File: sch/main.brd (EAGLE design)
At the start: 99.1 x 50.8 mm, 24 parts, among them IC2 PIC16F628P, T1 BC337, T2 BC337, T3 BC337

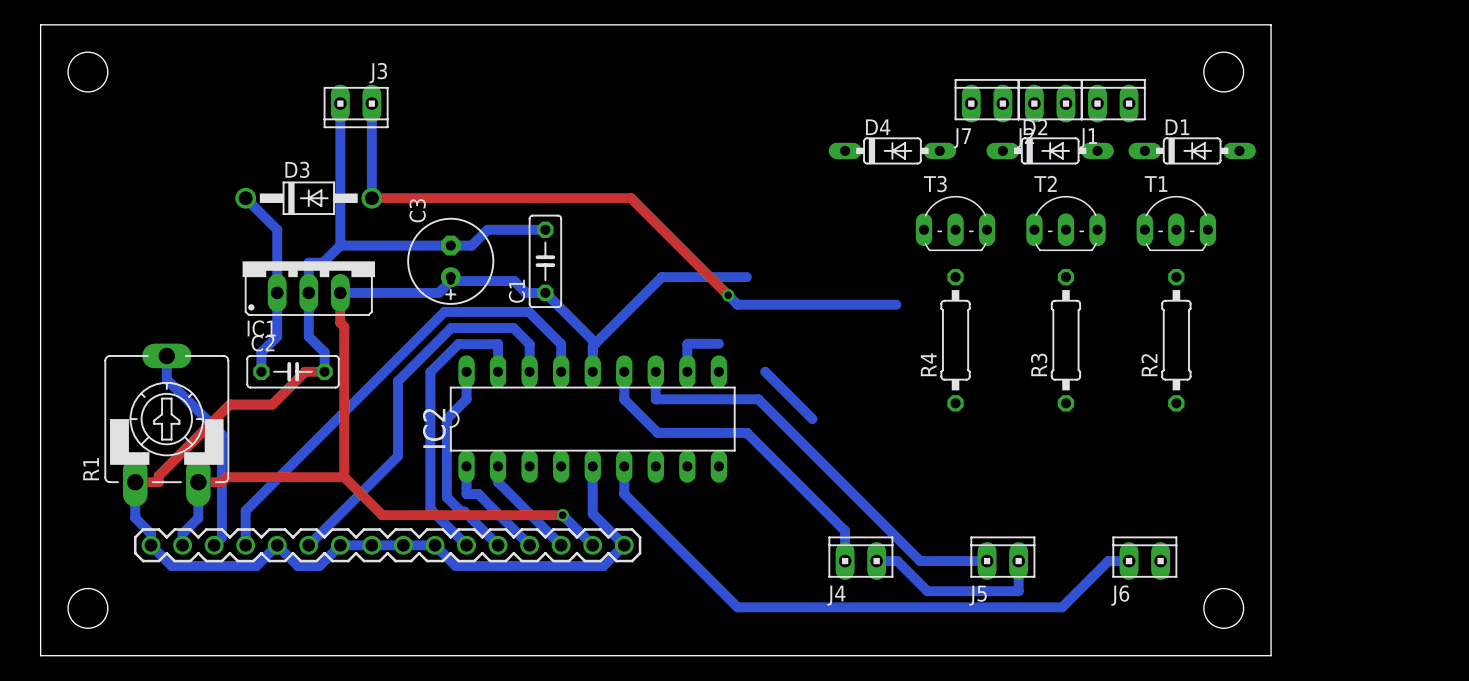
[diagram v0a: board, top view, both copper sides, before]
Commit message: First version for manufacturing
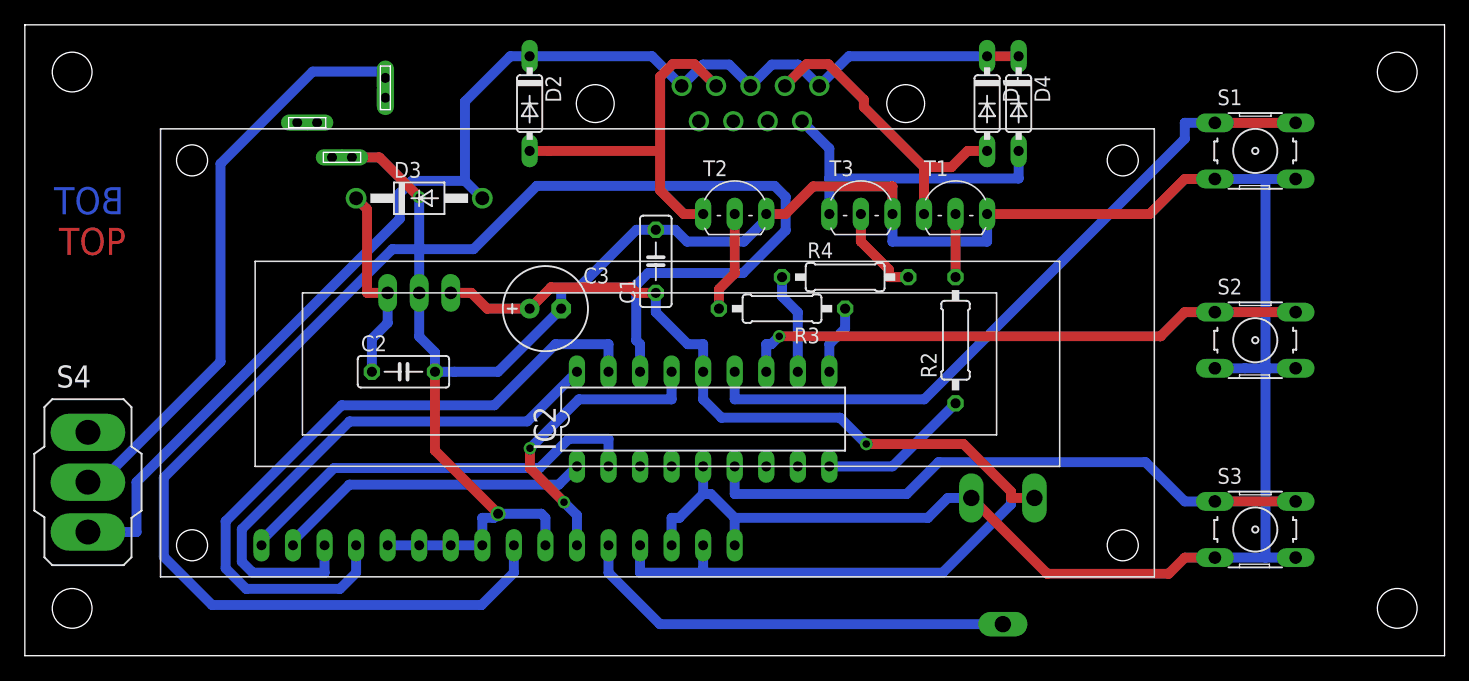
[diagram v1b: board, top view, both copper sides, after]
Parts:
- removed J1, J2, J3, J4, J5, J6, J7: (no value), con-amp:10X02MTA
- added S1, S2, S3: (no value), switch-omron:B3F-10XX
- added S4: (no value), switch:320-916
- added U1: LCD_BL_16X2_LOW, lcdmodules2:LCD_BL_16X2_LOW
- added X1: D-SUB9-H2M09ST, con-thomas-betts:H2M09ST
- U$1: value LCD_BL_16X2 -> KLDVX-0202-A; device lcdmodules:HEADER_16 -> con-kycon:KLDVX-0202-A
- moved R1 68.3 mm to (77.5, 7.62), flipped to the bottom, turned to 180 degrees
- moved D2 42.1 mm to (39.4, 44.5), turned to 270 degrees
- moved U$1 39.4 mm to (22.9, 45.7), flipped to the bottom
- moved T2 26.7 mm to (55.9, 35.6)
- moved R3 23.0 mm to (59.7, 27.9), turned to 180 degrees
- moved T1 17.8 mm to (73.7, 35.6)
- moved R2 17.8 mm to (73.7, 25.4)
- moved D1 16.9 mm to (76.2, 44.5), turned to 270 degrees
- moved D4 10.9 mm to (78.7, 44.5), turned to 270 degrees
- moved IC1 10.2 mm to (30.5, 26.7), flipped to the bottom, turned to 180 degrees
- moved R4 10.2 mm to (64.8, 30.5), turned to 0 degrees
- moved C1 8.89 mm to (49.5, 31.8)
- moved C2 8.89 mm to (29.2, 22.9)
- moved D3 8.89 mm to (30.5, 36.8)
- moved IC2 8.89 mm to (53.3, 19.1)
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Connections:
- new net N$12: S4.2, U$1.1
- net +12V: now also S4.3, X1.1, X1.3, X1.5; no longer J1.1, J2.1, J3.2, J7.1
- net +5V: now also U1.15, U1.2; no longer U$1.15, U$1.2
- net DB0: now also U1.11; no longer U$1.11
- net DB1: now also U1.12; no longer U$1.12
- net DB2: now also U1.13; no longer U$1.13
- net DB3: now also U1.14; no longer U$1.14
- net E: now also U1.6; no longer U$1.6
- net GND: now also S1.3, S1.4, S2.3, S2.4, S3.3, S3.4, U$1.2, U1.1, U1.10, U1.16, U1.5, U1.7, U1.8, U1.9; no longer J3.1, J4.1, J5.1, J6.1, U$1.1, U$1.10, U$1.16, U$1.5, U$1.7, U$1.8, U$1.9
- net N$11: now also U1.3; no longer U$1.3
- net N$2: now also X1.2; no longer J1.2
- net N$5: now also X1.4; no longer J2.2
- net N$9: now also X1.6; no longer J7.2
- net RS: now also U1.4; no longer U$1.4
- net SW1: now also S1.1, S1.2; no longer J4.2
- net SW2: now also S2.1, S2.2; no longer J5.2
- net SW3: now also S3.1, S3.2; no longer J6.2
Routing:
- net GND: track 130.2 -> 236.8 mm, vias 0 -> 2
- net E: track 31.3 -> 123.3 mm
- net +12V: track 53.4 -> 104.9 mm, vias 1 -> 0
- net N$12: track 0.00 -> 47.4 mm
- net DB0: track 23.7 -> 56.7 mm
- net SW1: track 26.8 -> 57.4 mm
- net N$5: track 0.00 -> 29.6 mm
- net DB1: track 16.5 -> 44.1 mm
- net N$9: track 0.00 -> 25.8 mm
- net DB3: track 8.45 -> 33.9 mm
- net N$2: track 0.00 -> 25.1 mm
- net N$11: track 17.3 -> 35.7 mm
- net DB2: track 9.01 -> 25.7 mm
- net RS: track 38.1 -> 24.6 mm, vias 0 -> 2
- net SW2: track 34.3 -> 45.9 mm, vias 0 -> 1
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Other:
- board size 99.1 x 50.8 mm -> 114.3 x 50.8 mm
- board text added: "BOT"
- board text added: "TOP"

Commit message: Updated 3d model
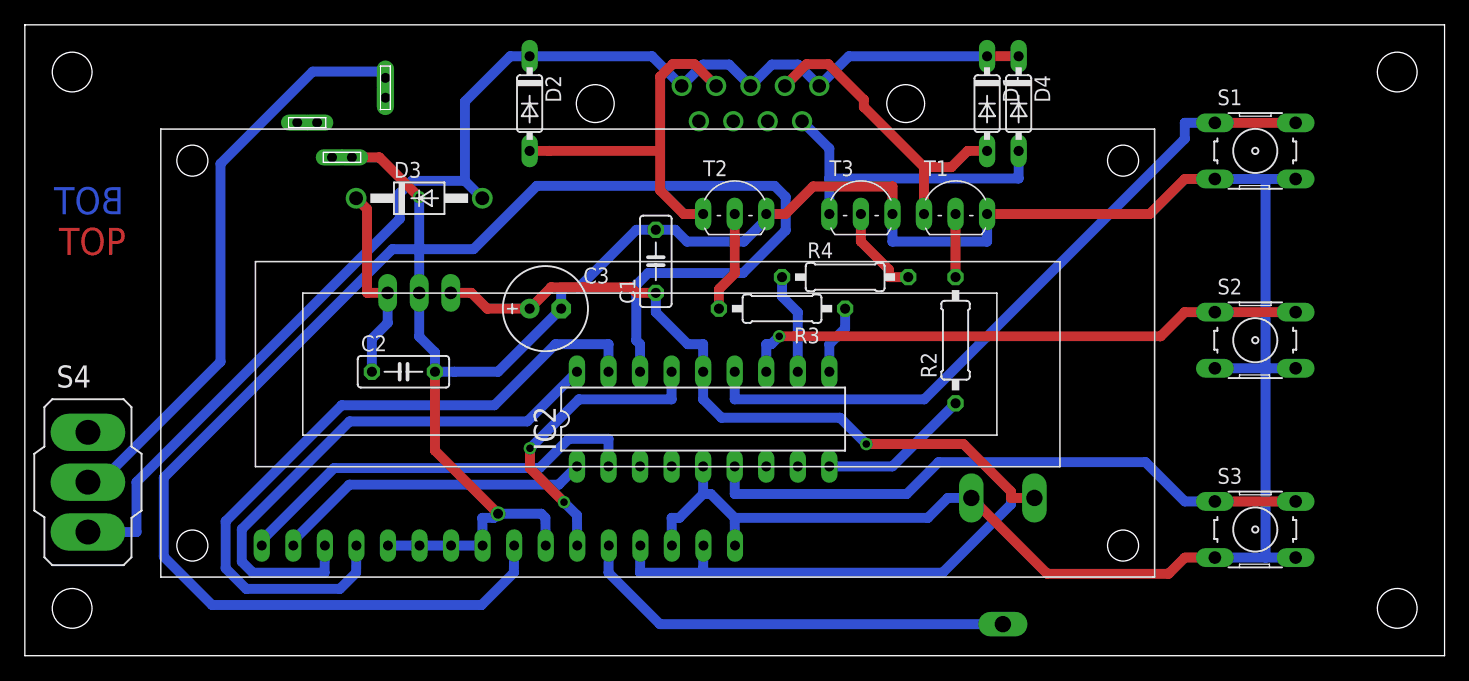
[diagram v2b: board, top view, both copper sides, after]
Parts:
- U1: value LCD_BL_16X2_LOW -> YM1602G_LOWCON; device lcdmodules2:LCD_BL_16X2_LOW -> lcdmodules2:YM1602G_LOWCON
- moved U1 34.9 mm to (48.9, 24.7)
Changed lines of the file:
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@@
 <?xml version="1.0" encoding="utf-8"?>
 <!DOCTYPE eagle SYSTEM "eagle.dtd">
-<eagle version="6.2">
+<eagle version="6.1">
 <drawing>
 <settings>
@@
 </element>
 <element name="S4" library="switch" package="320-916" value="" x="3.81" y="13.97"/>
-<element name="U1" library="lcdmodules2" package="LCD_BL_16X2_LOW" value="LCD_BL_16X2_LOW" x="17.78" y="8.89"/>
+<element name="U1" library="lcdmodules2" package="YM1602G_LOWCON" value="YM1602G_LOWCON" x="48.919590625" y="24.743953125"/>
 </elements>
 <signals>
@@
 <wire x1="98.6171" y1="23.1394" x2="98.6171" y2="38.3794" width="0.8" layer="16"/>
 <wire x1="101.0412" y1="38.3794" x2="98.6171" y2="38.3794" width="0.8" layer="16"/>
-<wire x1="98.6171" y1="23.1394" x2="96.9629" y2="23.1394" width="0.8" layer="16"/>
-<wire x1="94.5388" y1="23.1394" x2="96.9629" y2="23.1394" width="0.8" layer="16"/>
+<wire x1="94.5388" y1="23.1394" x2="98.6171" y2="23.1394" width="0.8" layer="16"/>
 <wire x1="98.6171" y1="7.8994" x2="94.5388" y2="7.8994" width="0.8" layer="16"/>
 <wire x1="101.0412" y1="7.8994" x2="98.6171" y2="7.8994" width="0.8" layer="16"/>
@@
 <wire x1="62.2014" y1="37.7809" x2="59.9805" y2="35.56" width="0.8" layer="1"/>
 <wire x1="94.5388" y1="7.8994" x2="92.1147" y2="7.8994" width="0.8" layer="1"/>
-<wire x1="50.8" y1="8.89" x2="50.8" y2="11.0981" width="0.8" layer="16"/>
+<wire x1="50.824590625" y1="8.868953125" x2="50.8" y2="11.0981" width="0.8" layer="16"/>
 <wire x1="50.8" y1="11.0981" x2="51.419" y2="11.0981" width="0.8" layer="16"/>
 <wire x1="51.419" y1="11.0981" x2="53.34" y2="13.0191" width="0.8" layer="16"/>
@@
 <wire x1="71.4374" y1="11.0981" x2="55.88" y2="11.0981" width="0.8" layer="16"/>
 <wire x1="53.34" y1="15.24" x2="53.34" y2="13.0191" width="0.8" layer="16"/>
-<wire x1="55.88" y1="8.89" x2="55.88" y2="11.0981" width="0.8" layer="16"/>
+<wire x1="55.904590625" y1="8.868953125" x2="55.88" y2="11.0981" width="0.8" layer="16"/>
 <wire x1="55.88" y1="11.0981" x2="53.959" y2="13.0191" width="0.8" layer="16"/>
 <wire x1="53.959" y1="13.0191" x2="53.34" y2="13.0191" width="0.8" layer="16"/>
@@
 <wire x1="31.75" y1="24.4205" x2="30.48" y2="25.6905" width="0.8" layer="16"/>
 <wire x1="30.48" y1="25.6905" x2="30.48" y2="29.21" width="0.8" layer="16"/>
-<wire x1="31.879" y1="22.86" x2="31.75" y2="22.86" width="0.8" layer="16"/>
-<wire x1="31.879" y1="22.86" x2="33.3105" y2="22.86" width="0.8" layer="16"/>
+<wire x1="31.75" y1="22.86" x2="33.3105" y2="22.86" width="0.8" layer="16"/>
 <wire x1="68.58" y1="35.56" x2="68.58" y2="33.3391" width="0.8" layer="16"/>
 <wire x1="76.2" y1="35.56" x2="76.2" y2="33.3391" width="0.8" layer="16"/>
@@
 <wire x1="47.9695" y1="34.29" x2="43.3197" y2="29.6402" width="0.8" layer="16"/>
 <wire x1="43.3197" y1="29.6402" x2="41.91" y2="29.6402" width="0.8" layer="16"/>
-<wire x1="40.64" y1="8.89" x2="40.64" y2="11.0981" width="0.8" layer="16"/>
-<wire x1="35.56" y1="8.89" x2="35.56" y2="11.0981" width="0.8" layer="16"/>
+<wire x1="40.664590625" y1="8.868953125" x2="40.64" y2="11.0981" width="0.8" layer="16"/>
+<wire x1="35.584590625" y1="8.868953125" x2="35.56" y2="11.0981" width="0.8" layer="16"/>
 <wire x1="35.56" y1="11.0981" x2="36.4981" y2="11.0981" width="0.8" layer="16"/>
 <wire x1="36.4981" y1="11.0981" x2="36.83" y2="11.43" width="0.8" layer="16"/>
-<wire x1="33.02" y1="8.89" x2="35.56" y2="8.89" width="0.8" layer="16"/>
+<wire x1="33.044590625" y1="8.868953125" x2="35.584590625" y2="8.868953125" width="0.8" layer="16"/>
 <via x="30.4665" y="36.9216" extent="1-16" drill="0.6096" diameter="1.016"/>
 <via x="36.83" y="11.43" extent="1-16" drill="0.8" diameter="1.2064"/>
@@
 <wire x1="36.83" y1="11.43" x2="40.3081" y2="11.43" width="0.8" layer="16"/>
 <wire x1="40.3081" y1="11.43" x2="40.64" y2="11.0981" width="0.8" layer="16"/>
-<wire x1="30.48" y1="8.89" x2="33.02" y2="8.89" width="0.8" layer="16"/>
-<wire x1="30.48" y1="8.89" x2="27.94" y2="8.89" width="0.8" layer="16"/>
+<wire x1="30.504590625" y1="8.868953125" x2="33.044590625" y2="8.868953125" width="0.8" layer="16"/>
+<wire x1="30.504590625" y1="8.868953125" x2="27.964590625" y2="8.868953125" width="0.8" layer="16"/>
 <wire x1="58.42" y1="35.56" x2="58.42" y2="35.1435" width="0.8" layer="16"/>
 <wire x1="58.42" y1="35.1435" x2="56.6156" y2="33.3391" width="0.8" layer="16"/>
@@
 <wire x1="78.1193" y1="12.1831" x2="78.1193" y2="12.7" width="0.8" layer="16"/>
 <wire x1="53.34" y1="7.007" x2="53.34" y2="6.6819" width="0.8" layer="16"/>
-<wire x1="53.34" y1="8.89" x2="53.34" y2="7.007" width="0.8" layer="16"/>
-<wire x1="48.26" y1="8.89" x2="48.26" y2="6.6819" width="0.8" layer="16"/>
+<wire x1="53.364590625" y1="8.868953125" x2="53.34" y2="7.007" width="0.8" layer="16"/>
+<wire x1="48.284590625" y1="8.868953125" x2="48.26" y2="6.6819" width="0.8" layer="16"/>
 <wire x1="53.34" y1="6.6819" x2="48.26" y2="6.6819" width="0.8" layer="16"/>
 <wire x1="39.37" y1="27.94" x2="35.9521" y2="27.94" width="0.8" layer="1"/>
@@
 <contactref element="U1" pad="11"/>
 <wire x1="45.72" y1="22.86" x2="45.72" y2="25.0809" width="0.8" layer="16"/>
-<wire x1="25.4" y1="8.89" x2="25.4" y2="6.6819" width="0.8" layer="16"/>
+<wire x1="25.424590625" y1="8.868953125" x2="25.4" y2="6.6819" width="0.8" layer="16"/>
 <wire x1="25.4" y1="6.6819" x2="24.0999" y2="5.3818" width="0.8" layer="16"/>
 <wire x1="24.0999" y1="5.3818" x2="16.5481" y2="5.3818" width="0.8" layer="16"/>
@@
 <contactref element="IC2" pad="18"/>
 <contactref element="U1" pad="12"/>
-<wire x1="22.86" y1="8.89" x2="22.86" y2="6.6819" width="0.8" layer="16"/>
+<wire x1="22.884590625" y1="8.868953125" x2="22.86" y2="6.6819" width="0.8" layer="16"/>
 <wire x1="22.86" y1="6.6819" x2="17.0866" y2="6.6819" width="0.8" layer="16"/>
 <wire x1="17.0866" y1="6.6819" x2="16.1944" y2="7.5741" width="0.8" layer="16"/>
@@
 <contactref element="IC2" pad="1"/>
 <contactref element="U1" pad="13"/>
-<wire x1="20.32" y1="8.89" x2="20.32" y2="9.2362" width="0.8" layer="16"/>
+<wire x1="20.344590625" y1="8.868953125" x2="20.32" y2="9.2362" width="0.8" layer="16"/>
 <wire x1="20.32" y1="9.2362" x2="24.854" y2="13.7702" width="0.8" layer="16"/>
 <wire x1="24.854" y1="13.7702" x2="41.7102" y2="13.7702" width="0.8" layer="16"/>
@@
 <contactref element="U1" pad="14"/>
 <wire x1="45.72" y1="15.24" x2="45.72" y2="17.4609" width="0.8" layer="16"/>
-<wire x1="17.78" y1="8.89" x2="17.78" y2="9.2617" width="0.8" layer="16"/>
+<wire x1="17.804590625" y1="8.868953125" x2="17.78" y2="9.2617" width="0.8" layer="16"/>
 <wire x1="17.78" y1="9.2617" x2="23.6261" y2="15.1078" width="0.8" layer="16"/>
 <wire x1="23.6261" y1="15.1078" x2="40.17" y2="15.1078" width="0.8" layer="16"/>
@@
 <contactref element="U1" pad="6"/>
 <wire x1="48.26" y1="22.86" x2="48.26" y2="25.0809" width="0.8" layer="16"/>
-<wire x1="38.1" y1="8.89" x2="38.1" y2="6.6819" width="0.8" layer="16"/>
+<wire x1="38.124590625" y1="8.868953125" x2="38.1" y2="6.6819" width="0.8" layer="16"/>
 <wire x1="38.1" y1="6.6819" x2="35.4998" y2="4.0817" width="0.8" layer="16"/>
 <wire x1="35.4998" y1="4.0817" x2="13.805" y2="4.0817" width="0.8" layer="16"/>
@@
 <wire x1="42.1372" y1="12.3586" x2="39.3961" y2="15.0997" width="0.8" layer="1"/>
 <wire x1="39.3961" y1="15.0997" x2="39.3961" y2="16.6997" width="0.8" layer="1"/>
-<wire x1="43.18" y1="8.89" x2="43.18" y2="11.3158" width="0.8" layer="16"/>
+<wire x1="43.204590625" y1="8.868953125" x2="43.18" y2="11.3158" width="0.8" layer="16"/>
 <wire x1="43.18" y1="11.3158" x2="42.1372" y2="12.3586" width="0.8" layer="16"/>
 <wire x1="50.8" y1="20.6391" x2="43.3355" y2="20.6391" width="0.8" layer="16"/>
@@
 <contactref element="R1" pad="S"/>
 <contactref element="U1" pad="3"/>
-<wire x1="45.72" y1="8.89" x2="45.72" y2="6.6819" width="0.8" layer="16"/>
+<wire x1="45.744590625" y1="8.868953125" x2="45.72" y2="6.6819" width="0.8" layer="16"/>
 <wire x1="45.72" y1="6.6819" x2="49.8619" y2="2.54" width="0.8" layer="16"/>
 <wire x1="49.8619" y1="2.54" x2="77.47" y2="2.54" width="0.8" layer="16"/>
